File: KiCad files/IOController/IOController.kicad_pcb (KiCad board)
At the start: 2 copper layers, 95.4 x 30 mm, 40 parts, among them IC1 TPS923654DMTR, J1 AVR-ISP-6, J101 Conn_01x04, J2 XT60 Horizontal Socket, J3 Conn_01x04, SW1 EC12, SW101 B3U, SW102 B3U, SW103 B3U, SW104 B3U, U1 AP7384-50SA, U2 ATtiny1634-M

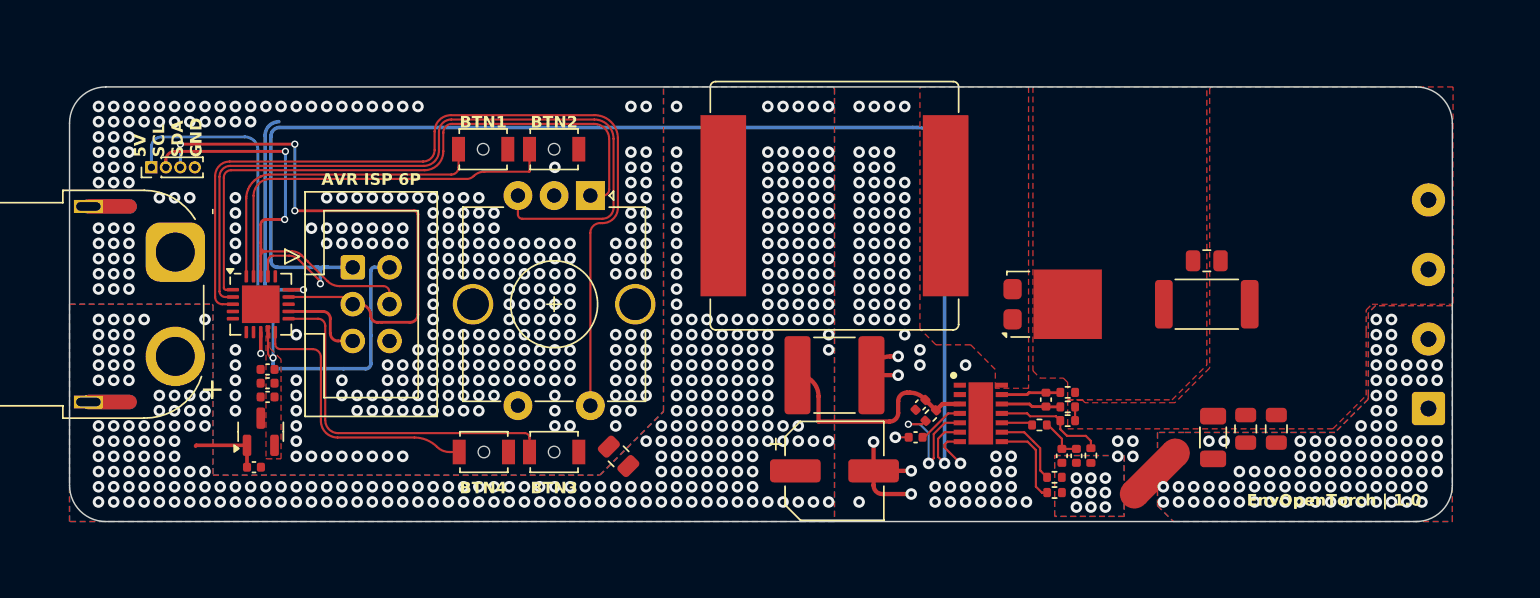
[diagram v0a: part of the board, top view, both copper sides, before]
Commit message: made a few small fixes.
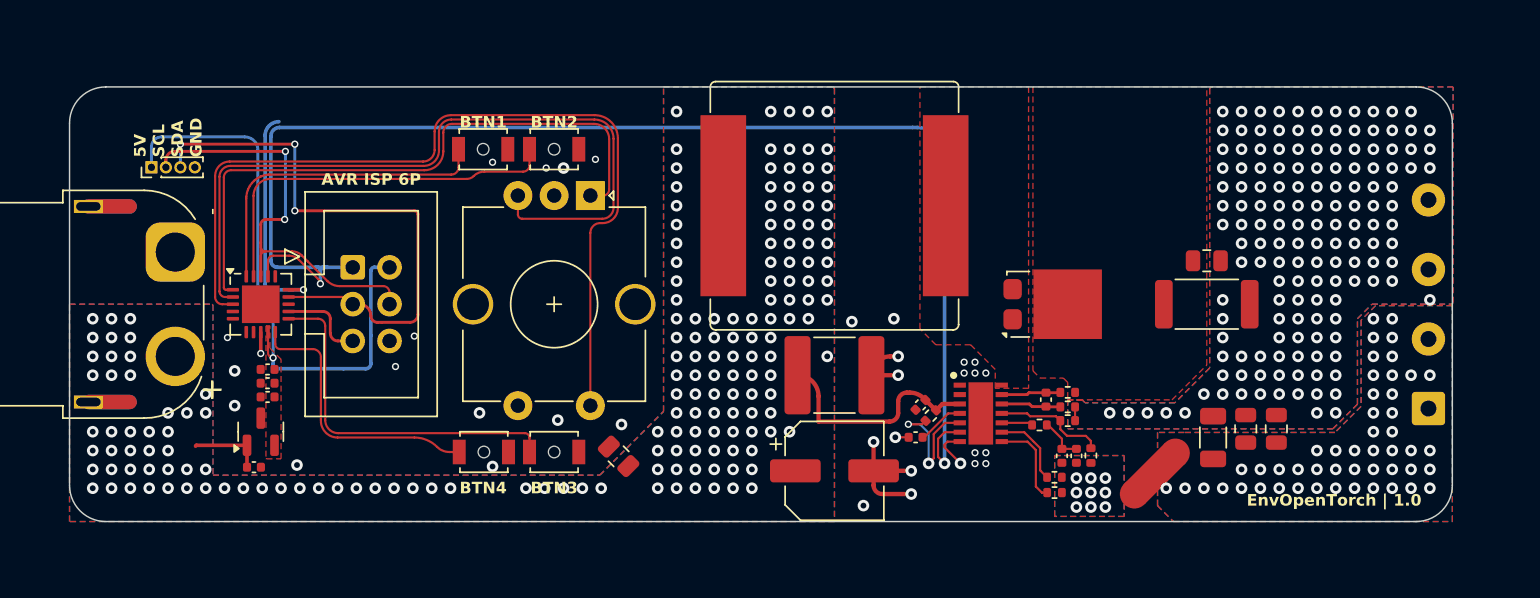
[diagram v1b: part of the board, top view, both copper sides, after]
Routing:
- net VCC: vias 310 -> 173
- net LED_V-: vias 95 -> 49
- net LED V+: vias 0 -> 147
- net GND: vias 376 -> 43
- added copper zone on B.Cu, net LED V+
